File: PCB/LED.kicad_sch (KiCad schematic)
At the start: 11 parts, among them Q2 2N7002

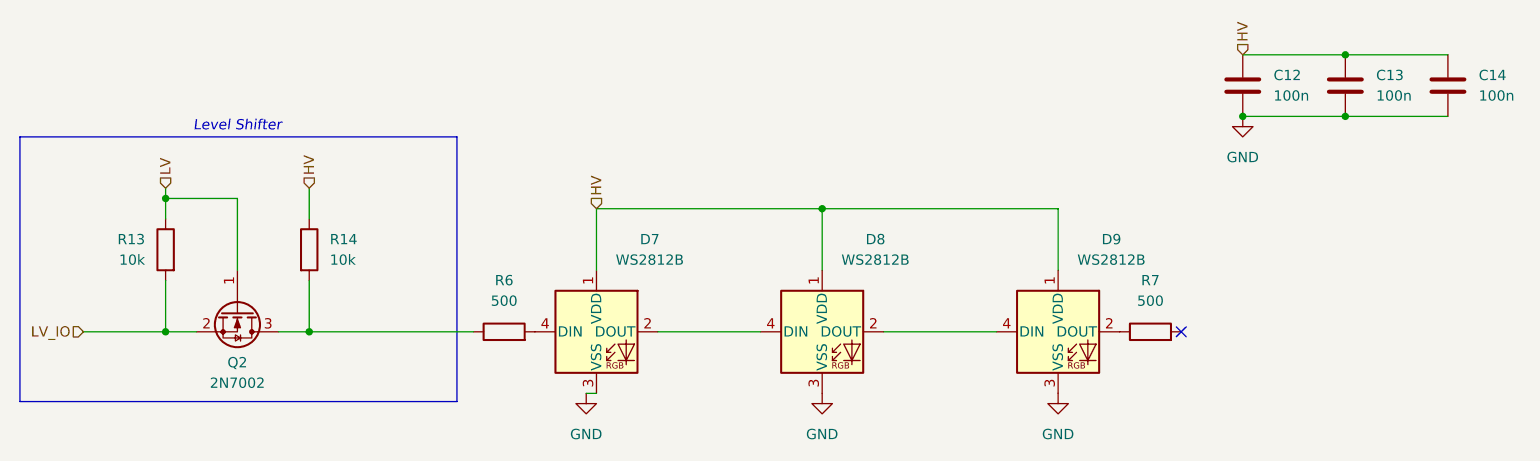
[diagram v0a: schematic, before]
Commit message: Initial Commit for INA219
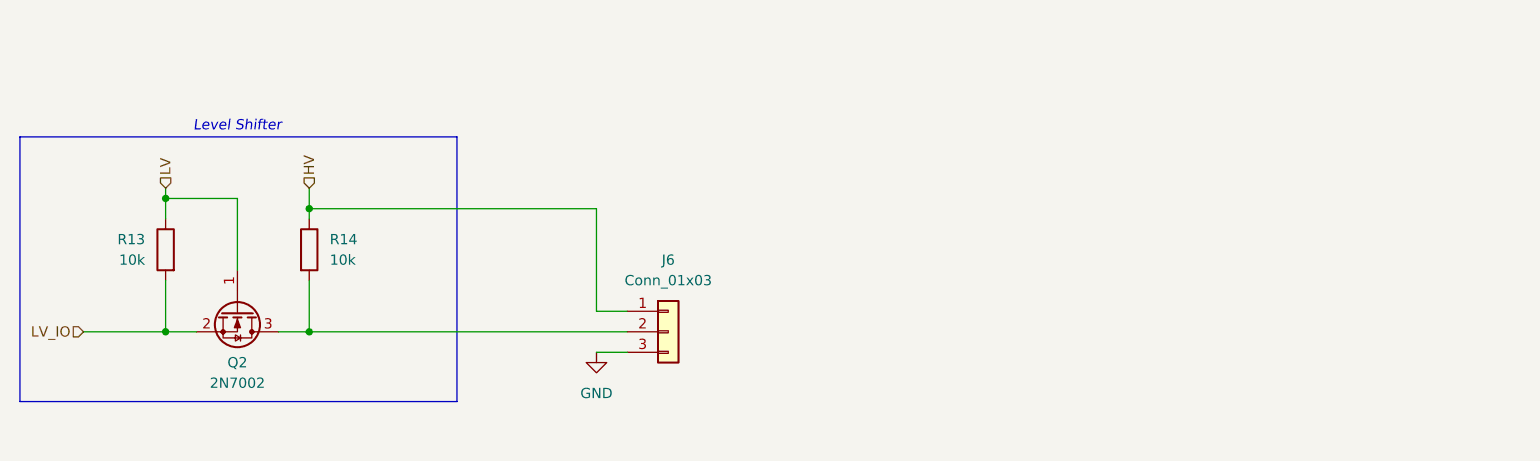
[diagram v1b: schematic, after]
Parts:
- removed C12, C13, C14: 100n, Capacitor_SMD:C_0402_1005Metric_Pad0.74x0.62mm_HandSolder, symbol Device:C
- removed D7, D8, D9: WS2812B, LED_SMD:LED_SK6812MINI_PLCC4_3.5x3.5mm_P1.75mm, symbol LED:WS2812B
- removed R6, R7: 500, Resistor_SMD:R_0402_1005Metric, symbol Device:R
- added J6: Conn_01x03, Connector_JST:JST_PH_S3B-PH-K_1x03_P2.00mm_Horizontal, symbol Connector_Generic:Conn_01x03
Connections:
- net GND: now also J6.3 (Pin_3)
- net HV: now also J6.1 (Pin_1)
- net at Q2.3 (D), R14.2: now also J6.2 (Pin_2)
- no-connect marks 1 -> 0
